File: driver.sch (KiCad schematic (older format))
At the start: 17 parts, among them IC1 L6205PD

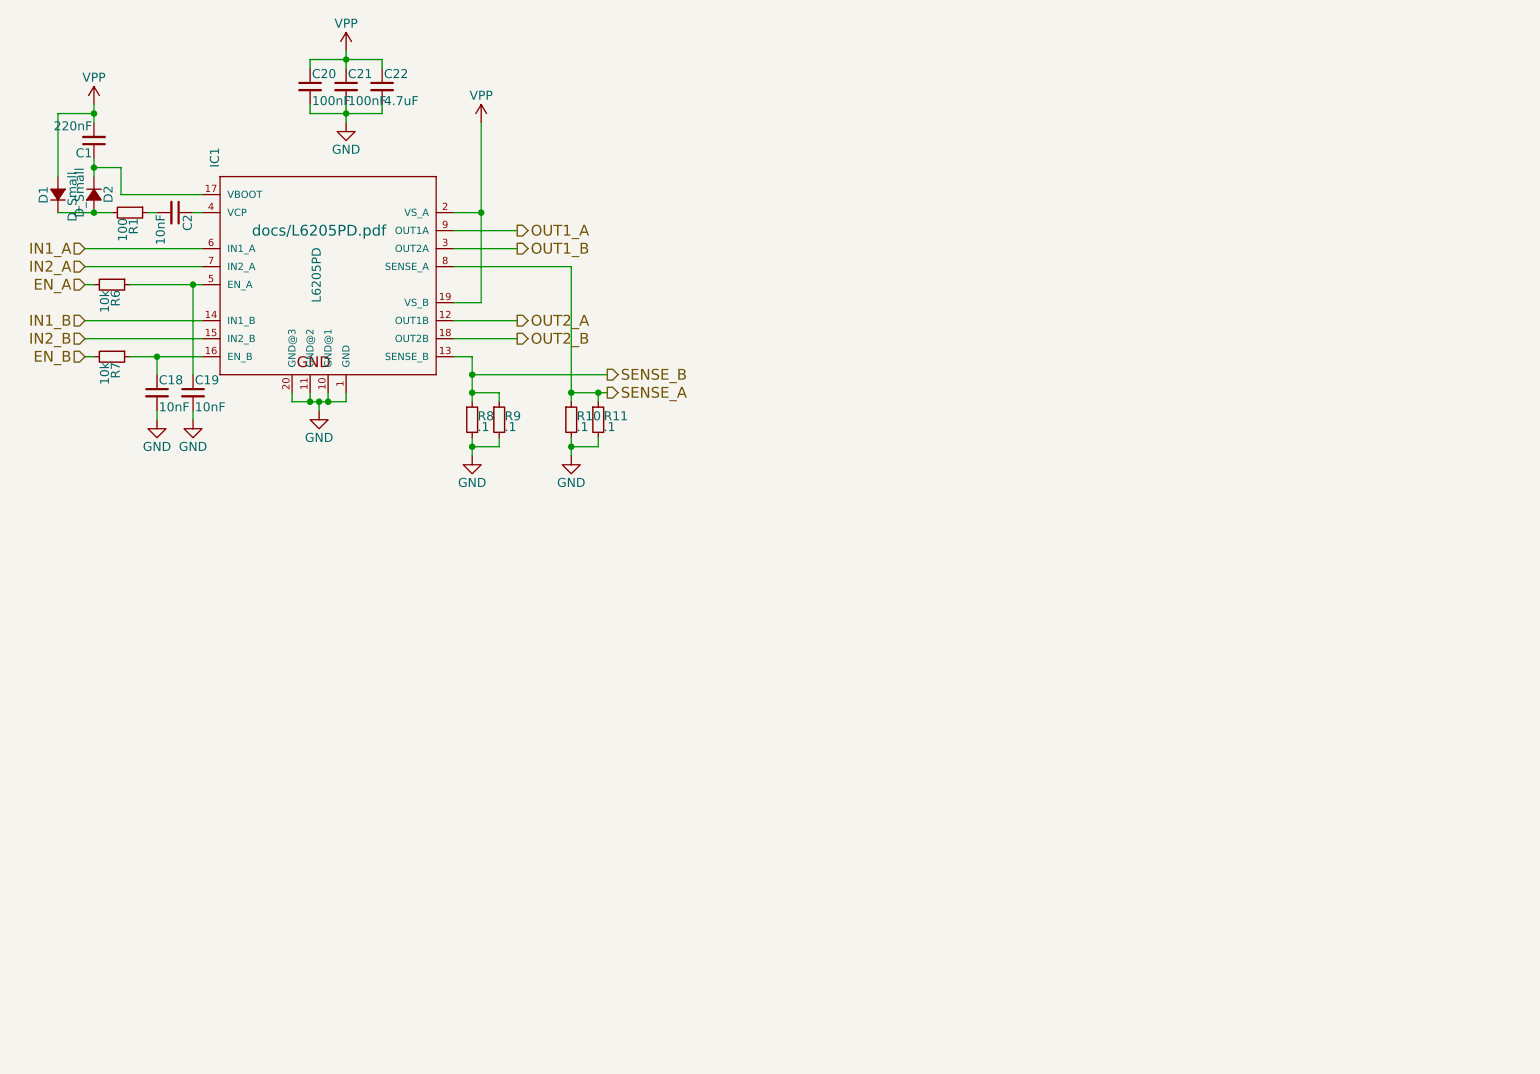
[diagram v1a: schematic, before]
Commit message: updated stuff
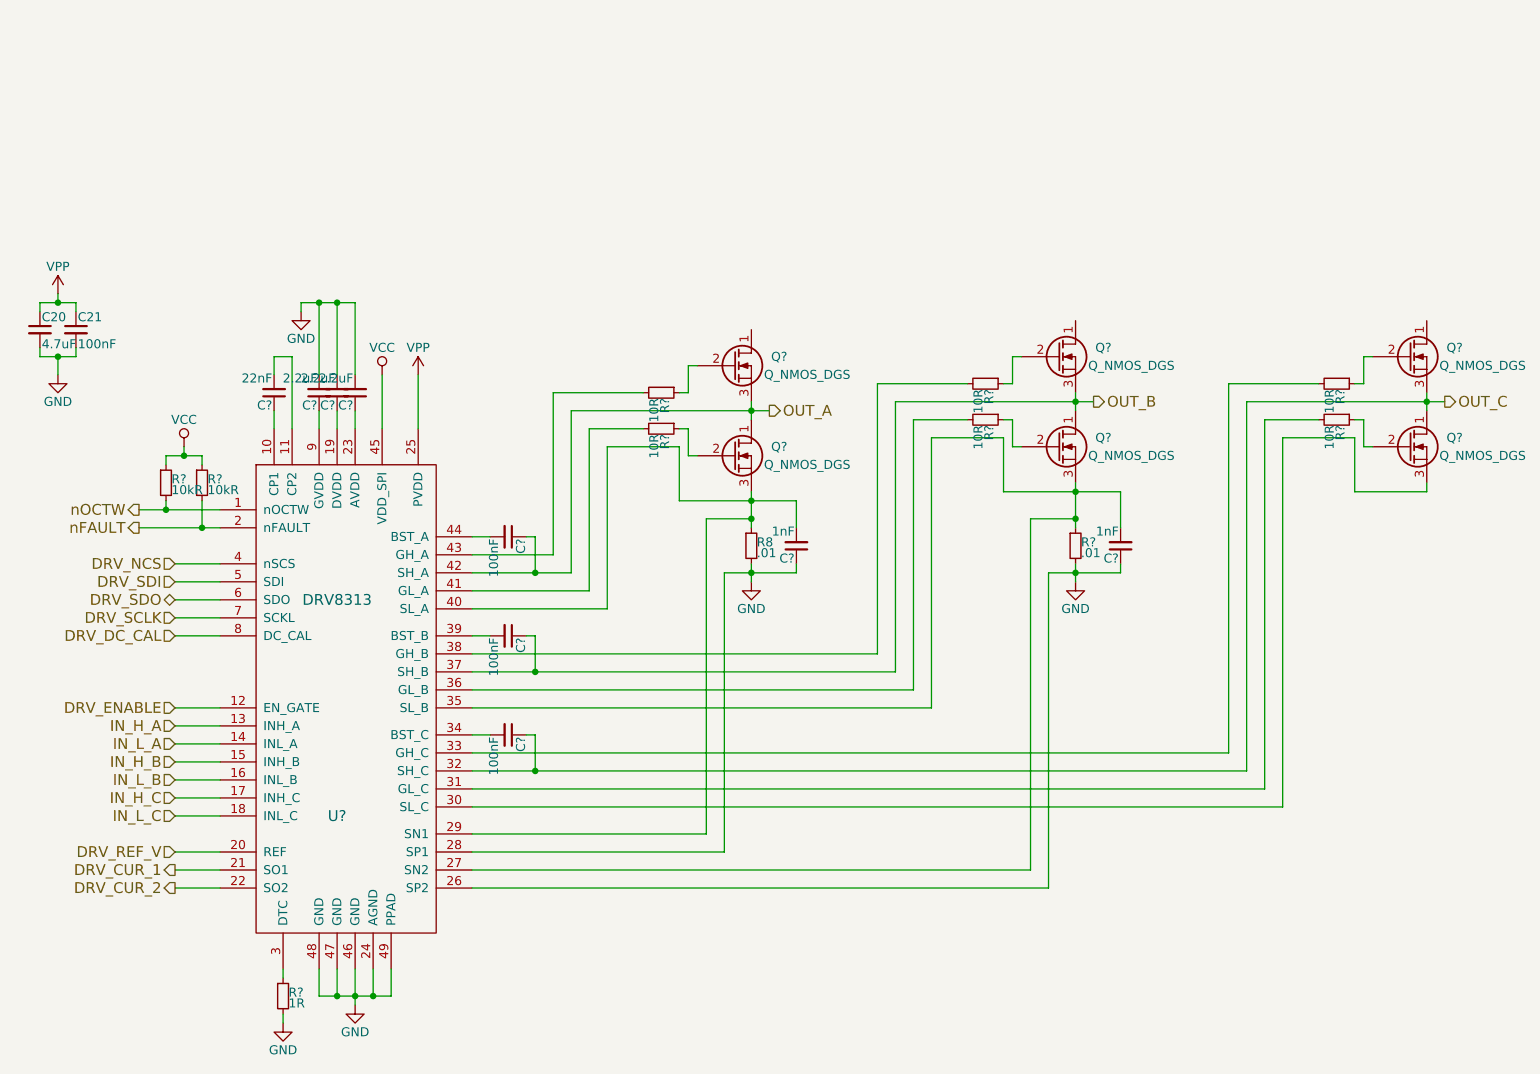
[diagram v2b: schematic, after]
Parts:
- removed C1: 220nF, Capacitors_SMD:C_0603, symbol C_Small
- removed C18, C19, C2: 10nF, Capacitors_SMD:C_0603, symbol C_Small
- removed C22: 4.7uF, Capacitors_SMD:C_0805, symbol C_Small
- removed D1, D2: D_Small, Diodes_SMD:SOD-323, symbol D_Small
- removed IC1: L6205PD, BLDC:SOIC-20, symbol L6205PD
- removed R1: 100, Resistors_SMD:R_0603, symbol R_Small
- removed R10, R11, R9: .1, Resistors_SMD:R_1206, symbol R_Small
- removed R6, R7: 10k, Resistors_SMD:R_0603, symbol R_Small
- added C? (x3): 2.2uF, Capacitors_SMD:C_0603, symbol C_Small
- added C? (x3): 100nF, Capacitors_SMD:C_0603, symbol C_Small
- added C? (x2): 1nF, Capacitors_SMD:C_0603, symbol C_Small
- added C?: 22nF, Capacitors_SMD:C_0603, symbol C_Small
- added Q? (x6): Q_NMOS_DGS, symbol Q_NMOS_DGS
- added R?: 1R, symbol R_Small
- added R? (x6): 10R, symbol R_Small
- added R?: .01, Resistors_SMD:R_1206, symbol R_Small
- added R? (x2): 10kR, symbol R_Small
- added U?: DRV8313, symbol DRV8313
- C20: value 100nF -> 4.7uF
- R8: value .1 -> .01
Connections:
- net GND: now also C?.1, C?.1, C?.2, C?.2, C?.2, R?.2, R?.2, U?.24 (AGND), U?.26 (SP2), U?.28 (SP1), U?.46 (GND), U?.47 (GND), U?.48 (GND), U?.49 (PPAD)
- net VPP: now also U?.25 (PVDD)
- net SENSE_B: no longer names the net of R8.1
- net SENSE_B: now also C?.2, Q?.3 (S), U?.29 (SN1), U?.40 (SL_A)
- new net: Q?.2 (G), R?.1 (x6)
- new net: C?.1, U?.9 (GVDD)
- new net: C?.1, U?.19 (DVDD)
- new net: C?.1, U?.23 (AVDD)
- new net: C?.1, U?.10 (CP1)
- new net: C?.2, U?.11 (CP2)
- new net: C?.2, Q?.3 (S), R?.1, U?.27 (SN2), U?.35 (SL_B)
- new net: R?.1, U?.3 (DTC)
- new net: Q?.3 (S), U?.30 (SL_C)
- new net: R?.2, U?.31 (GL_C)
- new net: R?.2, U?.33 (GH_C)
- new net: C?.2, U?.34 (BST_C)
- new net: R?.2, U?.36 (GL_B)
- new net: R?.2, U?.38 (GH_B)
- new net: C?.2, U?.39 (BST_B)
- new net: R?.2, U?.41 (GL_A)
- new net: R?.2, U?.43 (GH_A)
- new net: C?.2, U?.44 (BST_A)
- new net DRV_CUR_1: U?.21 (SO1)
- new net DRV_CUR_2: U?.22 (SO2)
- new net DRV_DC_CAL: U?.8 (DC_CAL)
- new net DRV_ENABLE: U?.12 (EN_GATE)
- new net DRV_NCS: U?.4 (nSCS)
- new net DRV_REF_V: U?.20 (REF)
- new net DRV_SCLK: U?.7 (SCKL)
- new net DRV_SDI: U?.5 (SDI)
- new net DRV_SDO: U?.6 (SDO)
- new net IN_H_A: U?.13 (INH_A)
- new net IN_H_B: U?.15 (INH_B)
- new net IN_H_C: U?.17 (INH_C)
- new net IN_L_A: U?.14 (INL_A)
- new net IN_L_B: U?.16 (INL_B)
- new net IN_L_C: U?.18 (INL_C)
- new net OUT_A: C?.1, Q?.1 (D), Q?.3 (S), U?.42 (SH_A)
- new net OUT_B: C?.1, Q?.1 (D), Q?.3 (S), U?.37 (SH_B)
- new net OUT_C: C?.1, Q?.1 (D), Q?.3 (S), U?.32 (SH_C)
- new net VCC: R?.1, R?.1, U?.45 (VDD_SPI)
- new net nFAULT: R?.2, U?.2 (nFAULT)
- new net nOCTW: R?.2, U?.1 (nOCTW)
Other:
- moved on the sheet: C20, C21, R8
